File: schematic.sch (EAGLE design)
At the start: 8 parts, among them J1 FTDI_DEVICE, U1 ATMEGA328P_TQFP

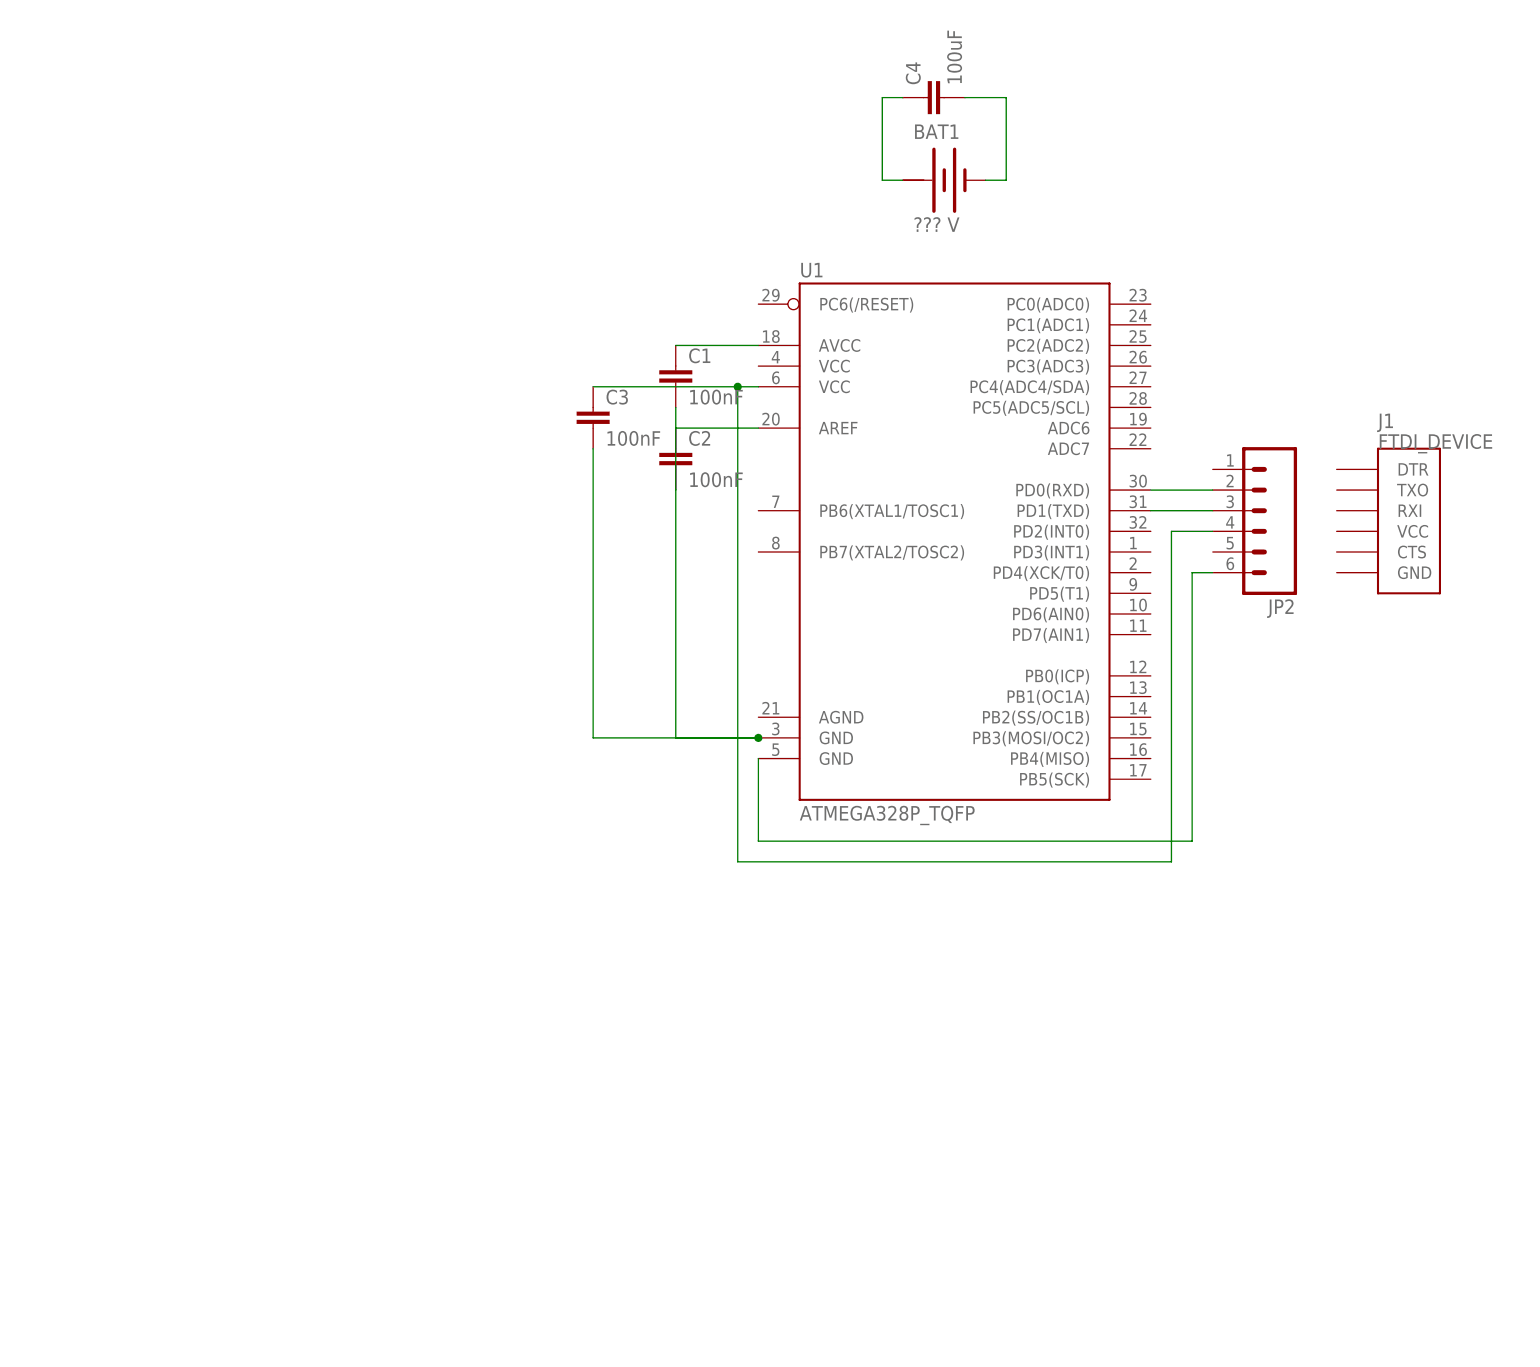
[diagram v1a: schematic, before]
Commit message: Added Will's changes
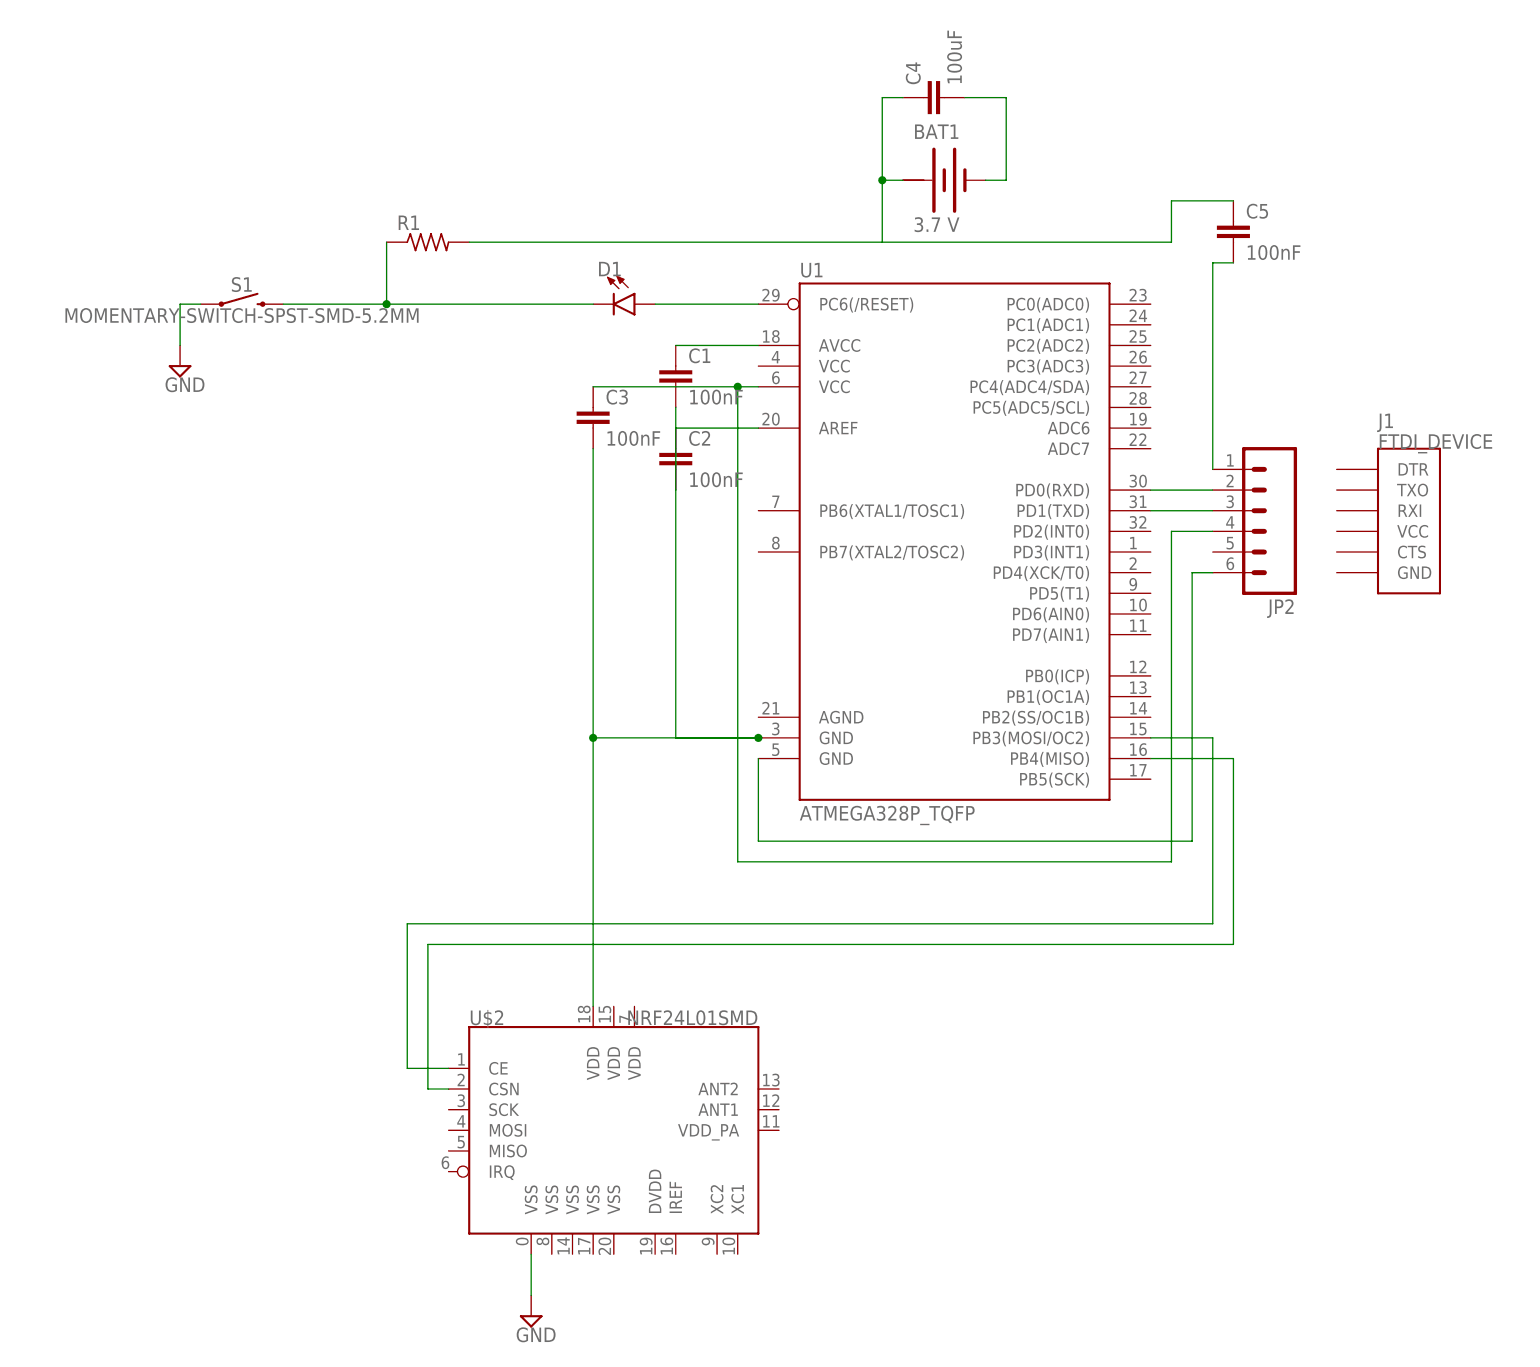
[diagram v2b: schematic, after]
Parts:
- added C5: 100nF, rcl:C-EUC0603
- added D1: (no value), SparkFun-LED:LED0603
- added R1: (no value), resistor:R-US_R0603
- added S1: MOMENTARY-SWITCH-SPST-SMD-5.2MM, SparkFun-Switches:MOMENTARY-SWITCH-SPST-SMD-5.2MM
- added U$2: NRF24L01SMD, SparkFun-RF:NRF24L01SMD
- BAT1: value ??? V -> 3.7 V
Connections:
- new net GND: S1.1, U$2.VSS@0
- new net N$10: C5.2, JP2.1
- new net N$11: C5.1, R1.2
- new net N$12: D1.A, U1.PC6(/RESET)
- new net N$13: D1.C, R1.1, S1.2
- new net N$14: U$2.CE, U1.PB3(MOSI/OC2)
- new net N$15: U$2.CSN, U1.PB4(MISO)
- net N$6: now also U$2.VDD@18
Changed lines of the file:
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@@
 <?xml version="1.0" encoding="utf-8"?>
 <!DOCTYPE eagle SYSTEM "eagle.dtd">
-<eagle version="8.4.3">
+<eagle version="8.4.1">
 <drawing>
 <settings>
@@
 <part name="C2" library="rcl" library_urn="urn:adsk.eagle:library:334" deviceset="C-EU" device="C0603" package3d_urn="urn:adsk.eagle:package:23616/2" value="100nF"/>
 <part name="C3" library="rcl" library_urn="urn:adsk.eagle:library:334" deviceset="C-EU" device="C0603" package3d_urn="urn:adsk.eagle:package:23616/2" value="100nF"/>
-<part name="BAT1" library="special" library_urn="urn:adsk.eagle:library:367" deviceset="BATTERY" device="" package3d_urn="urn:adsk.eagle:package:26670/1" value="??? V"/>
+<part name="BAT1" library="special" library_urn="urn:adsk.eagle:library:367" deviceset="BATTERY" device="" package3d_urn="urn:adsk.eagle:package:26670/1" value="3.7 V"/>
 <part name="C4" library="rcl" library_urn="urn:adsk.eagle:library:334" deviceset="C-EU" device="C2220K" package3d_urn="urn:adsk.eagle:package:23687/2" value="100uF"/>
 <part name="J1" library="quad" deviceset="FTDI_DEVICE" device=""/>
 <part name="JP2" library="SparkFun" deviceset="M06" device="SMD-FEMALE-V2"/>
+<part name="S1" library="SparkFun-Switches" deviceset="MOMENTARY-SWITCH-SPST" device="-SMD-5.2MM"/>
+<part name="SUPPLY1" library="supply2" library_urn="urn:adsk.eagle:library:372" deviceset="GND" device=""/>
+<part name="R1" library="resistor" library_urn="urn:adsk.eagle:library:348" deviceset="R-US_" device="R0603" package3d_urn="urn:adsk.eagle:package:26057/1"/>
+<part name="C5" library="rcl" library_urn="urn:adsk.eagle:library:334" deviceset="C-EU" device="C0603" package3d_urn="urn:adsk.eagle:package:23616/2" value="100nF"/>
+<part name="U$2" library="SparkFun-RF" deviceset="NRF24L01" device="SMD"/>
+<part name="SUPPLY2" library="supply2" library_urn="urn:adsk.eagle:library:372" deviceset="GND" device=""/>
+<part name="D1" library="SparkFun-LED" deviceset="LED" device="0603"/>
 </parts>
 <sheets>
@@
 <instance part="J1" gate="G$1" x="114.3" y="43.18"/>
 <instance part="JP2" gate="G$1" x="99.06" y="43.18" rot="R180"/>
+<instance part="S1" gate="G$1" x="-25.4" y="68.58"/>
+<instance part="SUPPLY1" gate="GND" x="-33.02" y="60.96"/>
+<instance part="R1" gate="G$1" x="-2.54" y="76.2"/>
+<instance part="C5" gate="G$1" x="96.52" y="78.74"/>
+<instance part="U$2" gate="G$1" x="20.32" y="-33.02"/>
+<instance part="SUPPLY2" gate="GND" x="10.16" y="-55.88"/>
+<instance part="D1" gate="G$1" x="22.86" y="68.58" rot="R270"/>
 </instances>
 <busses>
@@
 <wire x1="27.94" y1="55.88" x2="27.94" y2="45.72" width="0.1524" layer="91"/>
 <wire x1="27.94" y1="15.24" x2="38.1" y2="15.24" width="0.1524" layer="91"/>
+<pinref part="U$2" gate="G$1" pin="VDD@18"/>
+<wire x1="17.78" y1="15.24" x2="17.78" y2="-17.78" width="0.1524" layer="91"/>
+<junction x="17.78" y="15.24"/>
 </segment>
 </net>
@@
 <pinref part="BAT1" gate="G$1" pin="+"/>
 <wire x1="53.34" y1="83.82" x2="55.88" y2="83.82" width="0.1524" layer="91"/>
+<wire x1="53.34" y1="83.82" x2="53.34" y2="76.2" width="0.1524" layer="91"/>
+<junction x="53.34" y="83.82"/>
 </segment>
 </net>
@@
 </segment>
 </net>
+<net name="N$10" class="0">
+<segment>
+<pinref part="JP2" gate="G$1" pin="1"/>
+<pinref part="C5" gate="G$1" pin="2"/>
+<wire x1="93.98" y1="48.26" x2="93.98" y2="73.66" width="0.1524" layer="91"/>
+<wire x1="93.98" y1="73.66" x2="96.52" y2="73.66" width="0.1524" layer="91"/>
+</segment>
+</net>
+<net name="N$11" class="0">
+<segment>
+<pinref part="C5" gate="G$1" pin="1"/>
+<wire x1="96.52" y1="81.28" x2="88.9" y2="81.28" width="0.1524" layer="91"/>
+<wire x1="88.9" y1="81.28" x2="88.9" y2="76.2" width="0.1524" layer="91"/>
+<pinref part="R1" gate="G$1" pin="2"/>
+<wire x1="88.9" y1="76.2" x2="2.54" y2="76.2" width="0.1524" layer="91"/>
+</segment>
+</net>
+<net name="GND" class="0">
+<segment>
+<pinref part="S1" gate="G$1" pin="1"/>
+<pinref part="SUPPLY1" gate="GND" pin="GND"/>
+<wire x1="-30.48" y1="68.58" x2="-33.02" y2="68.58" width="0.1524" layer="91"/>
+<wire x1="-33.02" y1="68.58" x2="-33.02" y2="63.5" width="0.1524" layer="91"/>
+</segment>
+<segment>
+<pinref part="U$2" gate="G$1" pin="VSS@0"/>
+<wire x1="10.16" y1="-48.26" x2="10.16" y2="-53.34" width="0.1524" layer="91"/>
+<pinref part="SUPPLY2" gate="GND" pin="GND"/>
+</segment>
+</net>
+<net name="N$14" class="0">
+<segment>
+<pinref part="U1" gate="U$1" pin="PB3(MOSI/OC2)"/>
+<wire x1="86.36" y1="15.24" x2="93.98" y2="15.24" width="0.1524" layer="91"/>
+<wire x1="93.98" y1="15.24" x2="93.98" y2="-7.62" width="0.1524" layer="91"/>
+<wire x1="93.98" y1="-7.62" x2="-5.08" y2="-7.62" width="0.1524" layer="91"/>
+<pinref part="U$2" gate="G$1" pin="CE"/>
+<wire x1="-5.08" y1="-7.62" x2="-5.08" y2="-25.4" width="0.1524" layer="91"/>
+<wire x1="-5.08" y1="-25.4" x2="0" y2="-25.4" width="0.1524" layer="91"/>
+</segment>
+</net>
+<net name="N$15" class="0">
+<segment>
+<pinref part="U1" gate="U$1" pin="PB4(MISO)"/>
+<wire x1="86.36" y1="12.7" x2="96.52" y2="12.7" width="0.1524" layer="91"/>
+<wire x1="96.52" y1="12.7" x2="96.52" y2="-10.16" width="0.1524" layer="91"/>
+<wire x1="96.52" y1="-10.16" x2="-2.54" y2="-10.16" width="0.1524" layer="91"/>
+<wire x1="-2.54" y1="-10.16" x2="-2.54" y2="-27.94" width="0.1524" layer="91"/>
+<pinref part="U$2" gate="G$1" pin="CSN"/>
+<wire x1="-2.54" y1="-27.94" x2="0" y2="-27.94" width="0.1524" layer="91"/>
+</segment>
+</net>
+<net name="N$12" class="0">
+<segment>
+<pinref part="U1" gate="U$1" pin="PC6(/RESET)"/>
+<pinref part="D1" gate="G$1" pin="A"/>
+<wire x1="38.1" y1="68.58" x2="25.4" y2="68.58" width="0.1524" layer="91"/>
+</segment>
+</net>
+<net name="N$13" class="0">
+<segment>
+<pinref part="D1" gate="G$1" pin="C"/>
+<pinref part="S1" gate="G$1" pin="2"/>
+<wire x1="17.78" y1="68.58" x2="-7.62" y2="68.58" width="0.1524" layer="91"/>
+<pinref part="R1" gate="G$1" pin="1"/>
+<wire x1="-7.62" y1="68.58" x2="-20.32" y2="68.58" width="0.1524" layer="91"/>
+<wire x1="-7.62" y1="68.58" x2="-7.62" y2="76.2" width="0.1524" layer="91"/>
+<junction x="-7.62" y="68.58"/>
+</segment>
+</net>
